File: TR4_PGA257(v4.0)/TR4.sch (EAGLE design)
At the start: 131 parts, among them IC1 SN74AVC4T774PWR, IC3 SN74AVC4T774PWR, IC4 SN74AVC4T774PWR, IC7 LM1117IMPX-ADJ/NOPB, IC8 LM1117IMPX-ADJ/NOPB, IC9 LM1117IMPX-ADJ/NOPB, J4 2985-6004, J5 2985-6004, Q10 BSH103,235, Q11 BSH103,235, Q12 BSH103,235, Q13 BSH103,235, Q3 BSH103,235, Q4 BSH103,235, Q5 BSH103,235, Q6 BSH103,235, Q7 BSH103,235, Q8 BSH103,235, Q9 BSH103,235

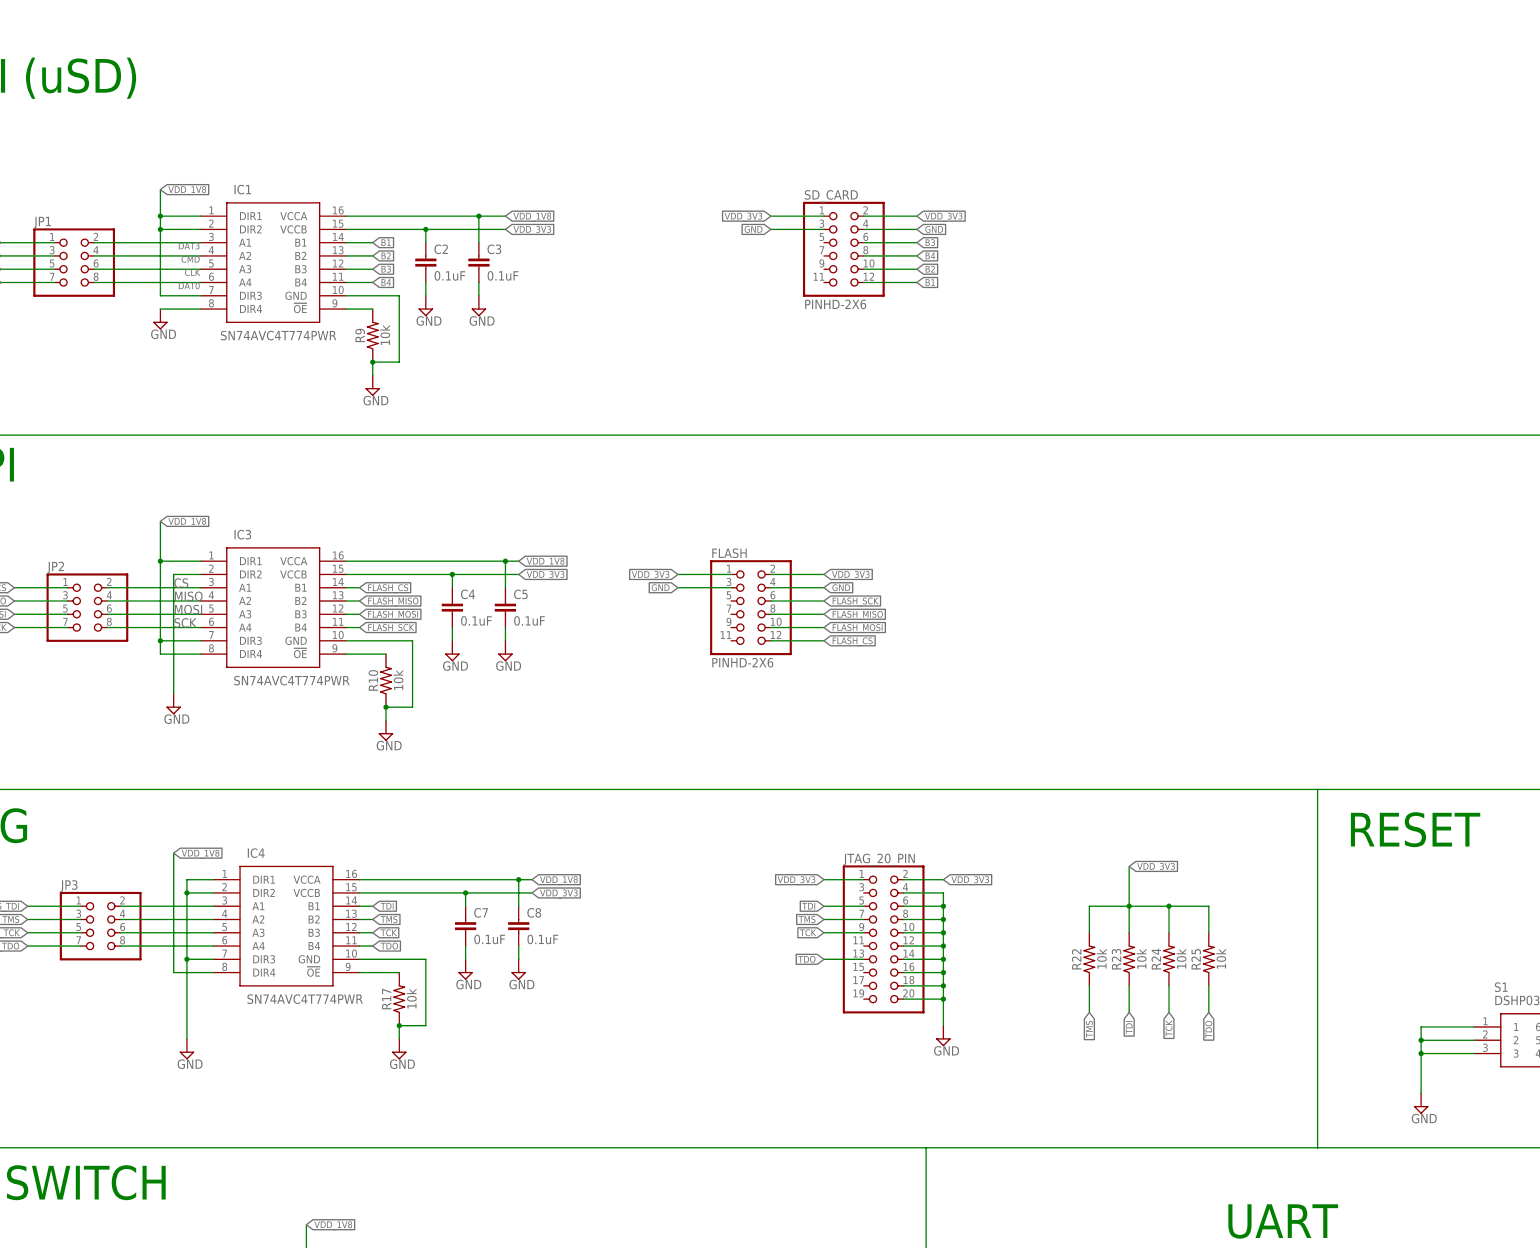
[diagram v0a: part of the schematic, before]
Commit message: update file
update BOM, position, and Gerber file, change the footprint of the level shifter
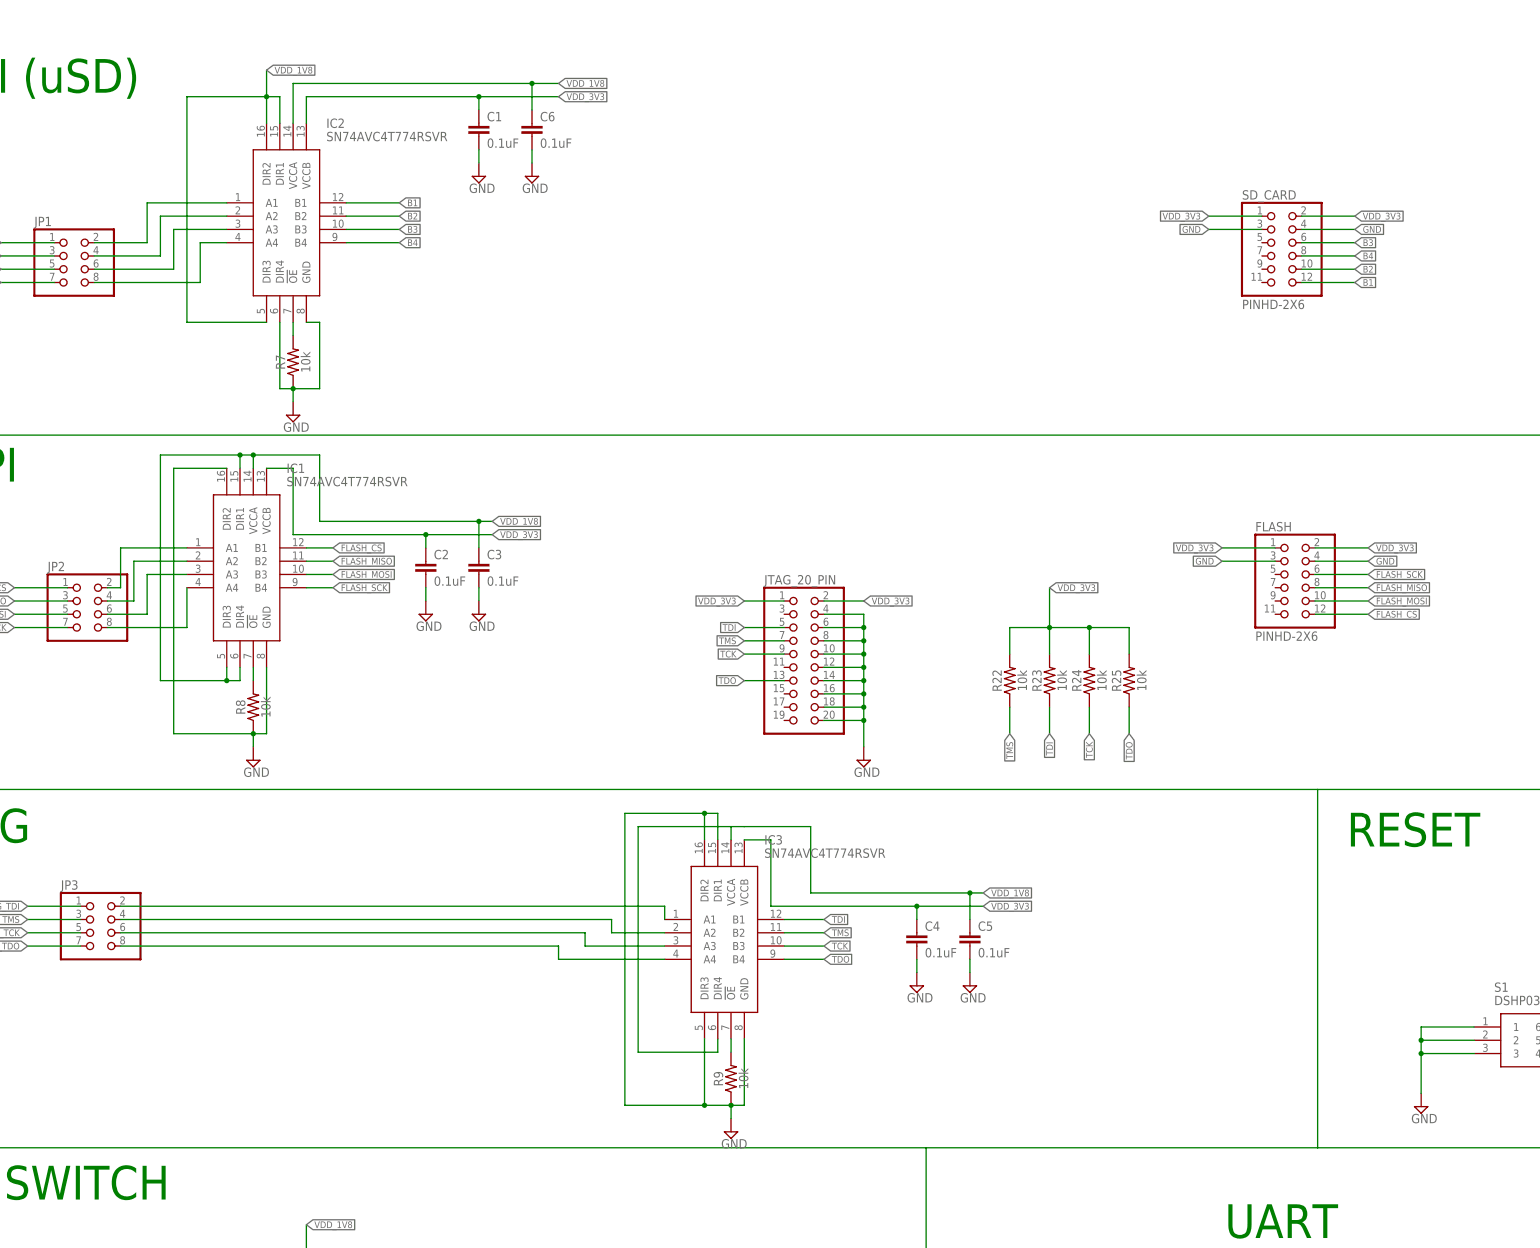
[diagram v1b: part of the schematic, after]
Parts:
- removed C7, C8: 0.1uF, SparkFun-Capacitors:0.1UF-0603-25V-5%
- removed IC4: SN74AVC4T774PWR, SamacSys_Parts:SN74AVC4T774PWR
- removed R10, R17: 10k, SparkFun-Resistors:10KOHM-0603-1/10W-1%
- added C1, C6: 0.1uF, SparkFun-Capacitors:0.1UF-0603-25V-5%
- added IC2: SN74AVC4T774RSVR, SamacSys_Parts:SN74AVC4T774RSVR
- added R7, R8: 10k, SparkFun-Resistors:10KOHM-0603-1/10W-1%
- IC1, IC3: value SN74AVC4T774PWR -> SN74AVC4T774RSVR; device SamacSys_Parts:SN74AVC4T774PWR -> SamacSys_Parts:SN74AVC4T774RSVR
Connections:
- removed net CLK: IC1.A3, JP1.6
- removed net CMD: IC1.A2, JP1.4
- removed net CS: IC3.A1, JP2.2
- removed net DAT0: IC1.A4, JP1.8
- removed net DAT3: IC1.A1, JP1.2
- removed net MISO: IC3.A2, JP2.4
- removed net MOSI: IC3.A3, JP2.6
- removed net N$16: IC4.!OE, R17.2
- removed net SCK: IC3.A4, JP2.8
- new net N$1: IC2.!OE, R7.2
- new net N$11: IC1.A1, JP2.2
- new net N$2: IC2.A1, JP1.2
- new net N$25: IC3.!OE, R9.2
- new net N$3: IC2.A2, JP1.4
- new net N$5: IC2.A3, JP1.6
- new net N$6: IC2.A4, JP1.8
- new net N$7: IC1.!OE, R8.2
- new net N$8: IC1.A4, JP2.8
- net B1: now also IC2.B1; no longer IC1.B1
- net B2: now also IC2.B2; no longer IC1.B2
- net B3: now also IC2.B3; no longer IC1.B3
- net B4: now also IC2.B4; no longer IC1.B4
- net FLASH_CS: now also IC1.B1; no longer IC3.B1
- net FLASH_MISO: now also IC1.B2; no longer IC3.B2
- net FLASH_MOSI: now also IC1.B3; no longer IC3.B3
- net FLASH_SCK: now also IC1.B4; no longer IC3.B4
- net GND: now also C1.2, C6.2, IC1.DIR2, IC2.DIR4, IC2.GND, IC3.DIR1, IC3.DIR3, R7.1, R8.1; no longer C7.2, C8.2, IC1.DIR4, IC4.DIR1, IC4.DIR2, IC4.DIR3, IC4.GND, R10.1, R17.1
- net N$10: now also IC1.A2, JP2.4; no longer IC3.!OE, R10.2
- net N$12: now also IC3.A1; no longer IC4.A1
- net N$13: now also IC3.A2; no longer IC4.A2
- net N$14: now also IC3.A3; no longer IC4.A3
- net N$15: now also IC3.A4; no longer IC4.A4
- net N$9: now also IC1.A3, JP2.6; no longer IC1.!OE, R9.2
- net TCK: now also IC3.B3; no longer IC4.B3
- net TDI: now also IC3.B1; no longer IC4.B1
- net TDO: now also IC3.B4; no longer IC4.B4
- net TMS: now also IC3.B2; no longer IC4.B2
- net VDD_1V8: now also C6.1, IC1.DIR4, IC2.DIR1, IC2.DIR2, IC2.DIR3, IC2.VCCA; no longer C8.1, IC1.DIR2, IC3.DIR1, IC3.DIR3, IC4.DIR4, IC4.VCCA
- net VDD_3V3: now also C1.1, IC2.VCCB; no longer C7.1, IC4.VCCB
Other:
- moved on the sheet: C2, C3, C4, C5, FLASH, IC1, IC3, JTAG_20_PIN, R22, R23, R24, R25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
